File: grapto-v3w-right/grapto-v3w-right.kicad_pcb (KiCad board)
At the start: 2 copper layers, 150 x 124.7 mm, 59 parts

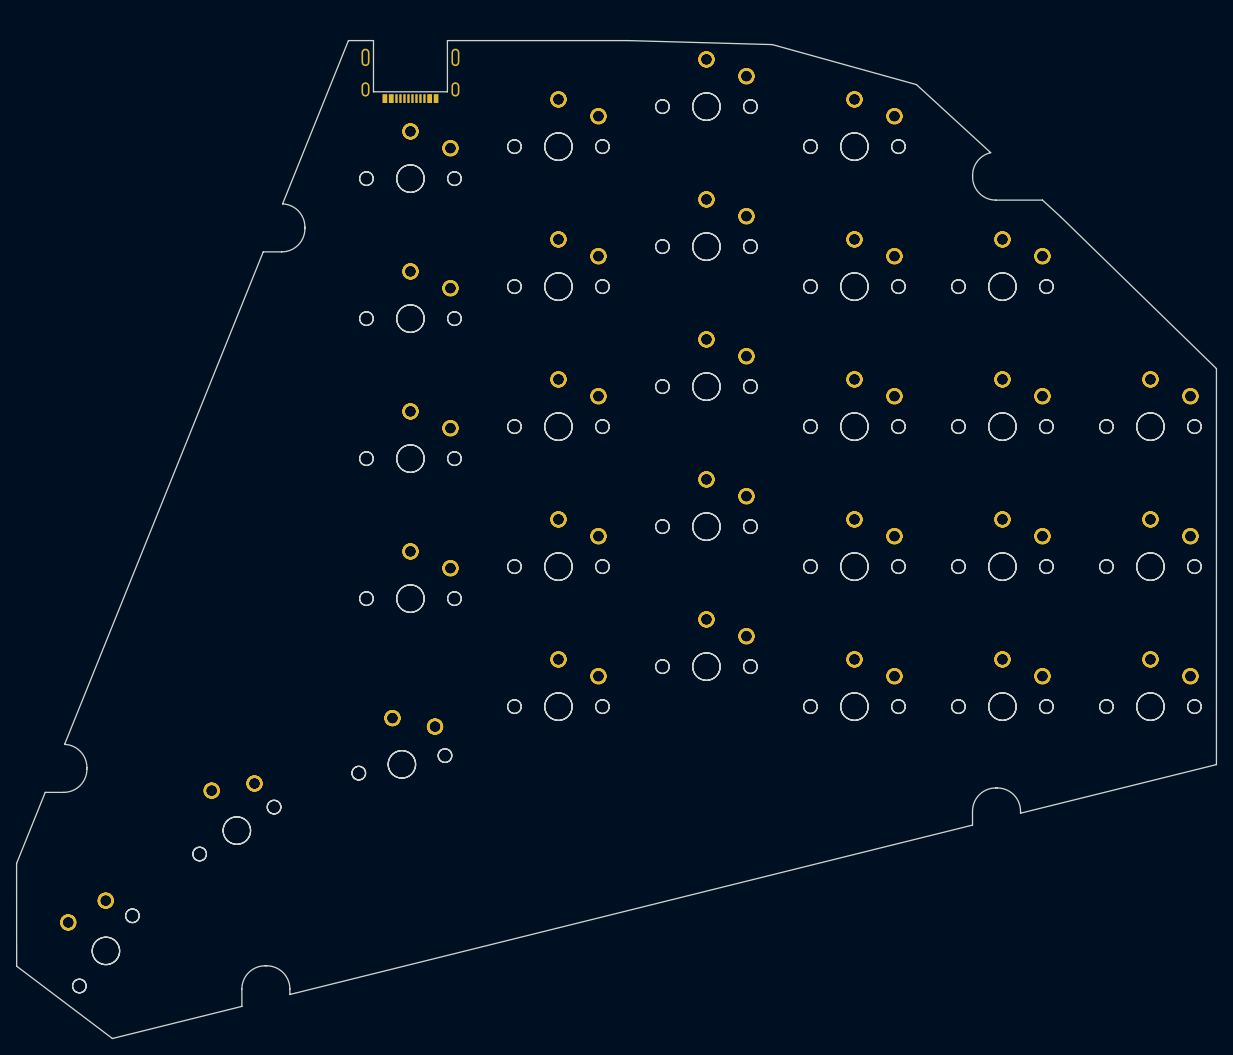
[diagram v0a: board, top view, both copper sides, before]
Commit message: update generated pcbs
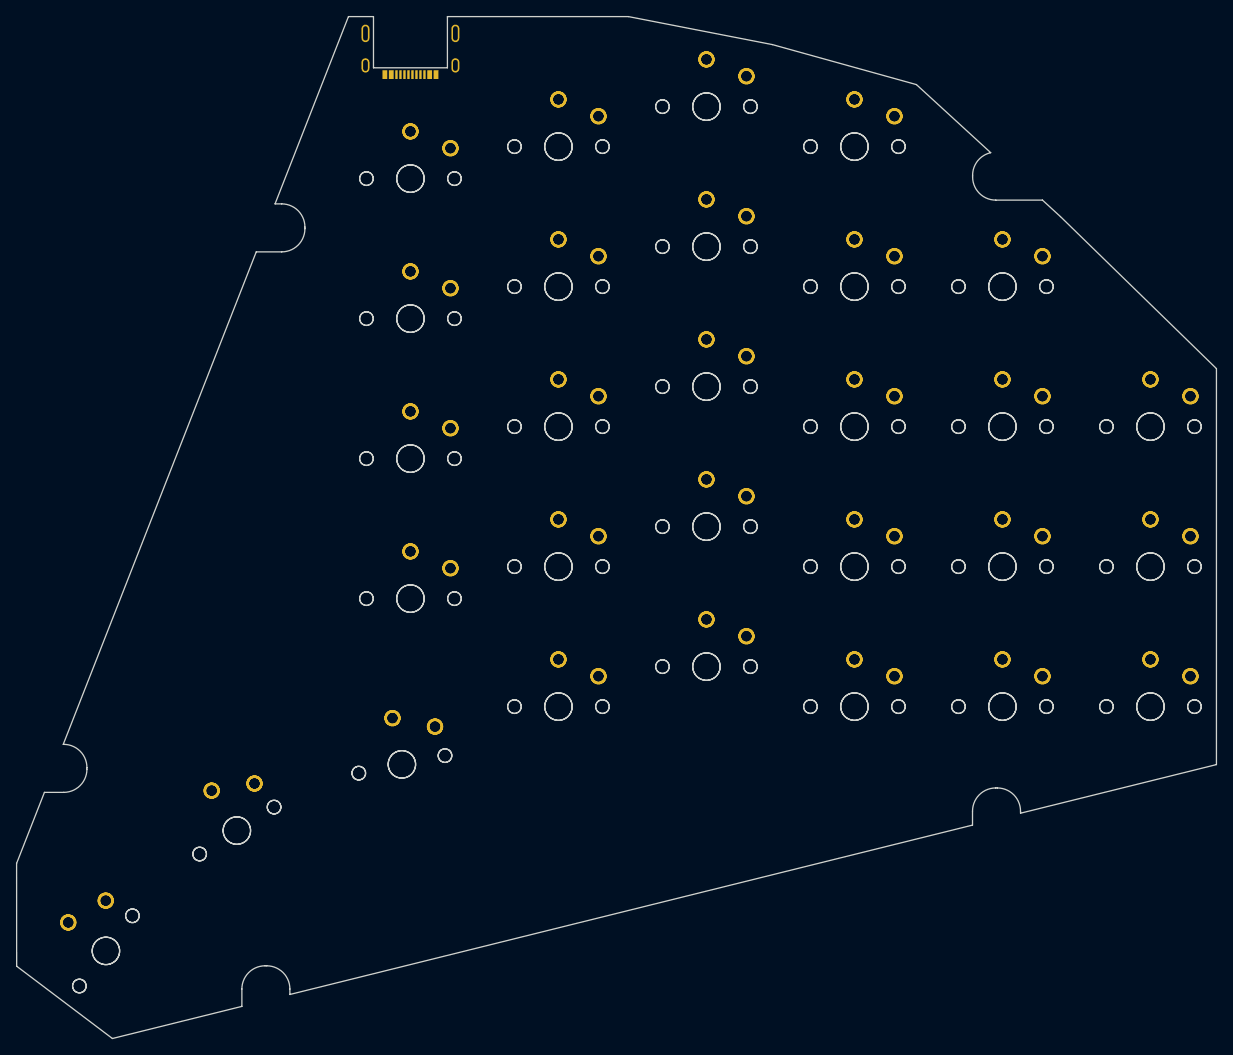
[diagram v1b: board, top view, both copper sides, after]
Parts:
- moved USBC1 3.00 mm to (129.0, 93.8)
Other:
- board size 150 x 124.7 mm -> 150 x 127.7 mm
